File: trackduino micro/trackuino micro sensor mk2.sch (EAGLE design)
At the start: 43 parts, among them IC2 74AHC1G125DBV, SW1 SPST_TACT-KMR2, U1 ATMEGA168MLF, Y1 16MHZ

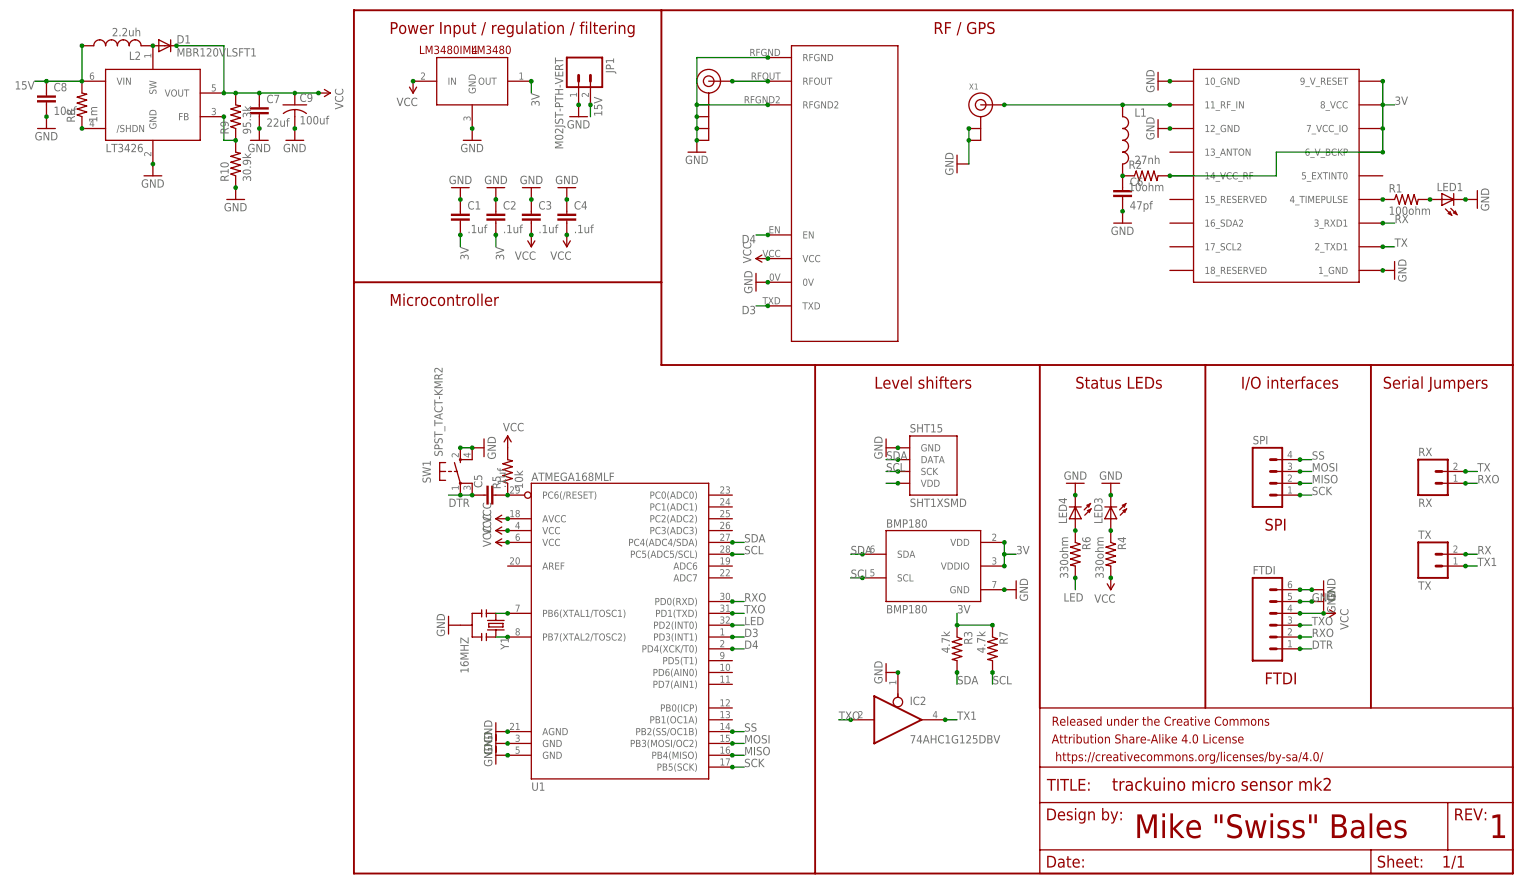
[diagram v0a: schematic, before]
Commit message: firmware
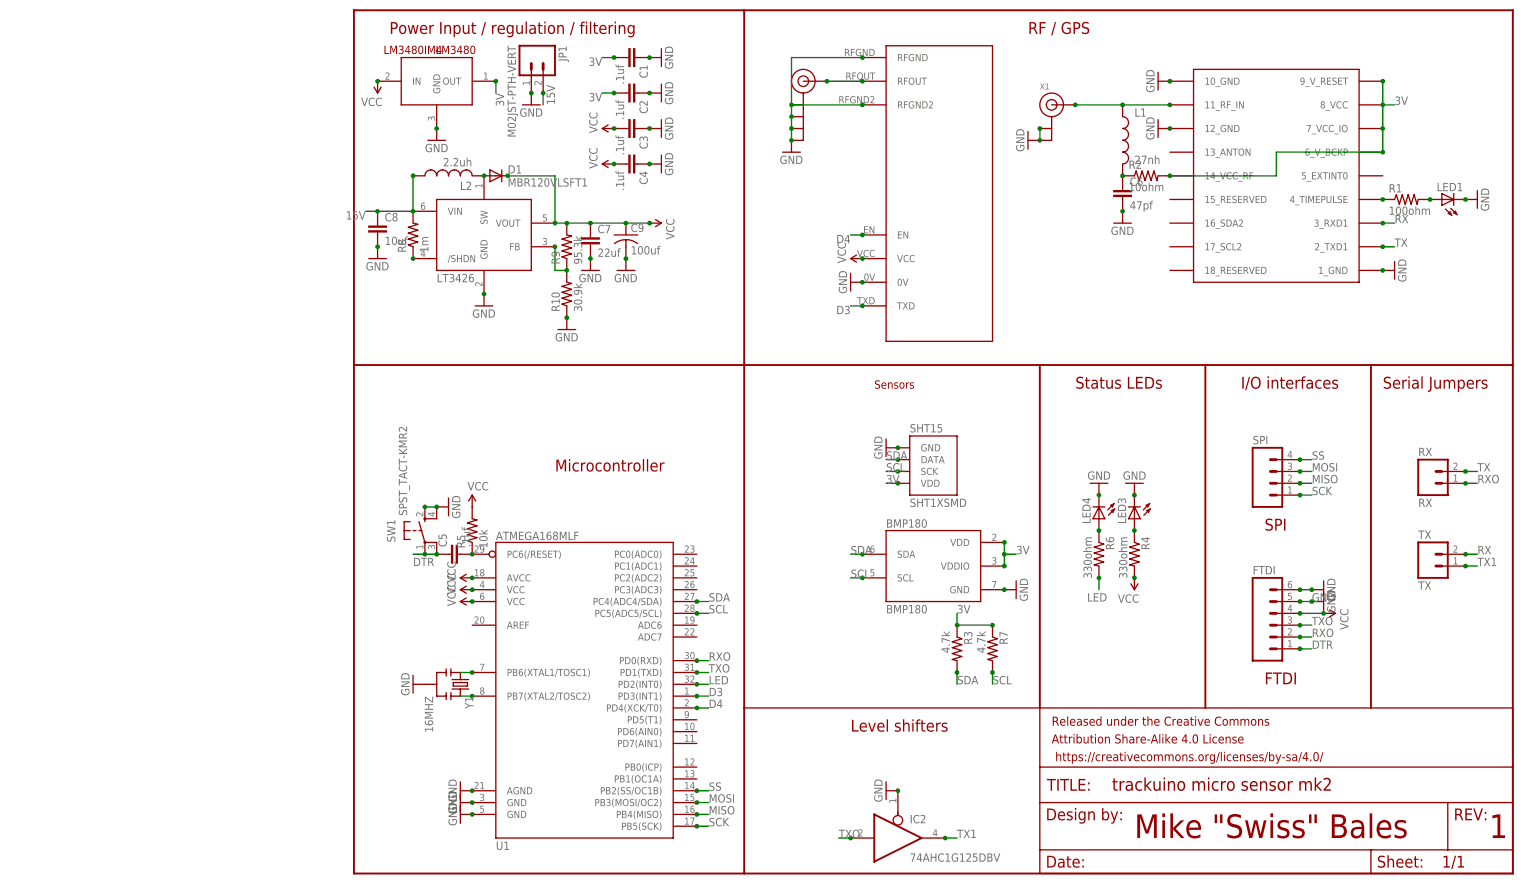
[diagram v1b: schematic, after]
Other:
- note added: "Sensors"
- moved on the sheet: C1, C2, C3, C4, C5, C7, C8, C9, D1, IC2, JP1, L2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
